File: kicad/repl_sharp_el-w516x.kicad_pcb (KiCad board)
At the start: 2 copper layers, 68.6 x 141.2 mm, 129 parts, among them J1 USB_B_Micro, J2 AVR-ISP-6, SW1 SW_RESET, SW10 SW_Push, SW12 SW_Push, SW14 SW_Push, SW15 SW_Push, SW16 SW_Push, SW17 SW_Push, SW18 SW_Push, SW19 SW_Push, SW21 SW_Push, SW22 SW_Push, SW23 SW_Push, SW24 SW_Push, SW25 SW_Push, SW26 SW_Push, SW28 SW_Push, SW3 SW_Push, SW30 SW_Push, SW31 SW_Push, SW32 SW_Push, SW33 SW_Push, SW34 SW_Push, SW35 SW_Push, SW36 SW_Push, SW37 SW_Push, SW38 SW_Push, SW39 SW_Push, SW4 SW_Push, SW40 SW_Push, SW41 SW_Push, SW42 SW_Push, SW43 SW_Push, SW44 SW_Push, SW45 SW_Push, SW46 SW_Push, SW47 SW_Push, SW5 SW_Push, SW50 SW_Push, SW51 SW_Push, SW52 SW_Push, SW53 SW_Push, SW54 SW_Push, SW55 SW_Push, SW58 SW_Push, SW59 SW_Push, SW6 SW_Push, SW60 SW_Push, SW61 SW_Push, SW62 SW_Push, SW63 SW_Push, SW66 SW_POWER, SW7 SW_Push, SW8 SW_Push, SW9 SW_Push, U1 SOIC-16_3.9x9.9mm_P1.27mm, U2 ATmega32U4-AU, U3 74HC595, U4 BQ24072RGTR, U5 AP2210-33, Y1 Crystal

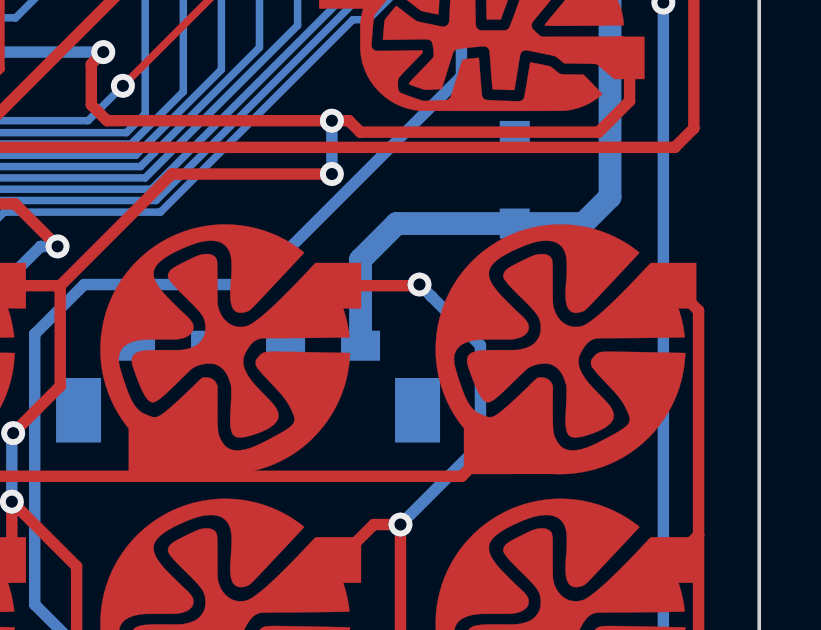
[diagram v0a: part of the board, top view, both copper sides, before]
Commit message: kicad: finalize device BOM
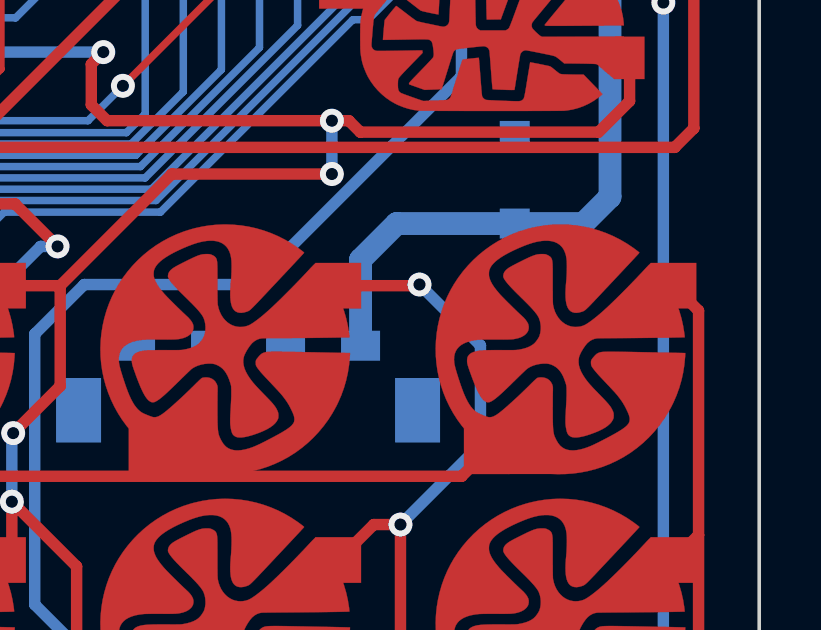
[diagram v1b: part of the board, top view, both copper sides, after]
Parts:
- U1: value SOIC-16_3.9x9.9mm_P1.27mm -> 74HC165D
